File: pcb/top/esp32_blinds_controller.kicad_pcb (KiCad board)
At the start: 2 copper layers, 100 x 68.2 mm, 28 parts, among them J1 Conn_01x05_Pin, K1 LEG-24, K2 LEG-24, K3 LEG-24, K4 LEG-24, U1 MCP23008-xP, U2 ULN2003A, U3 LTV-847

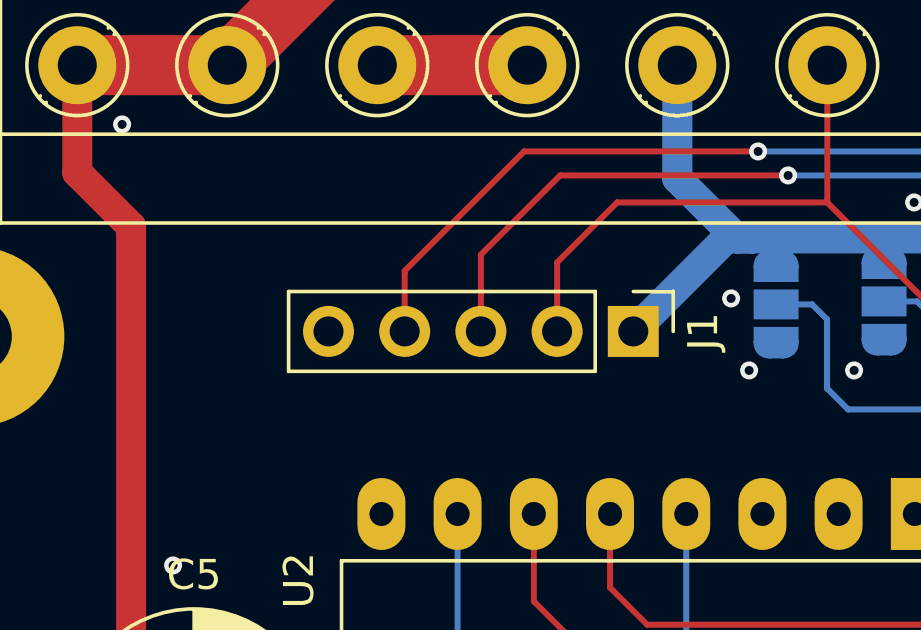
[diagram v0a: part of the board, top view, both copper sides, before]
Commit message: update
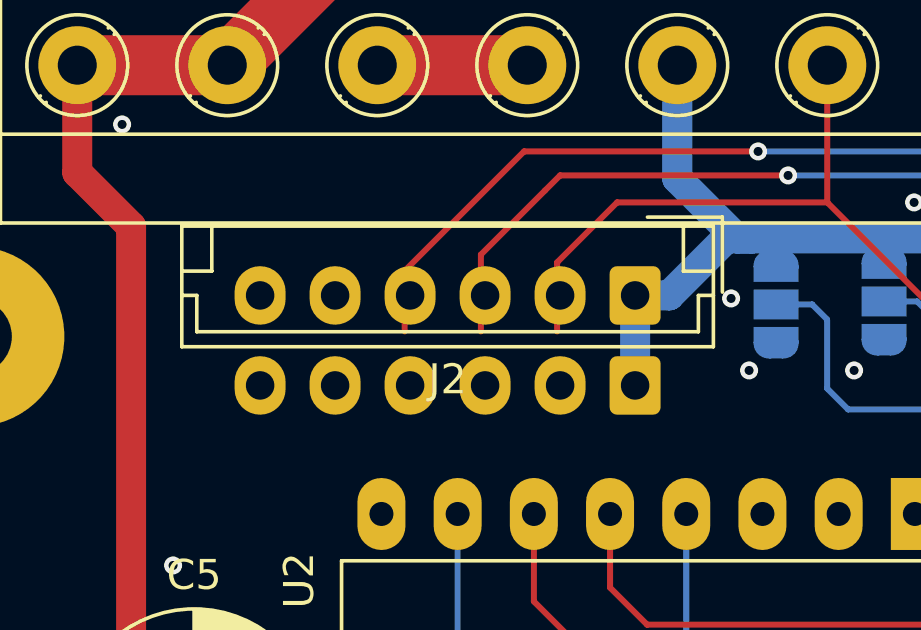
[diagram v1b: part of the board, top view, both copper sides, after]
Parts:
- added J2: Conn_01x05_Pin, Connector_JST:JST_EH_B6B-EH-A_1x06_P2.50mm_Vertical, F.Cu at (127.2, 76.0)
- J1: footprint Connector_PinHeader_2.54mm:PinHeader_1x05_P2.54mm_Vertical -> Connector_JST:JST_EH_B6B-EH-A_1x06_P2.50mm_Vertical; moved to B.Cu
- moved J1 1.80 mm to (127.2, 79.0), turned to 180 degrees
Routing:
- net +3V3: track 84.1 -> 86.5 mm
